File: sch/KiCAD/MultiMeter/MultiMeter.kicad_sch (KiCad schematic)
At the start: 28 parts, among them J1 Conn_01x02_Male, J2 Conn_01x02_Male, J3 Conn_01x03_Male, J4 Conn_01x03_Male, J5 Conn_01x02_Female, J6 Conn_01x15, J7 Conn_01x15, J8 Conn_01x08_Female, Q1 2SC1815, Q2 2SC1815

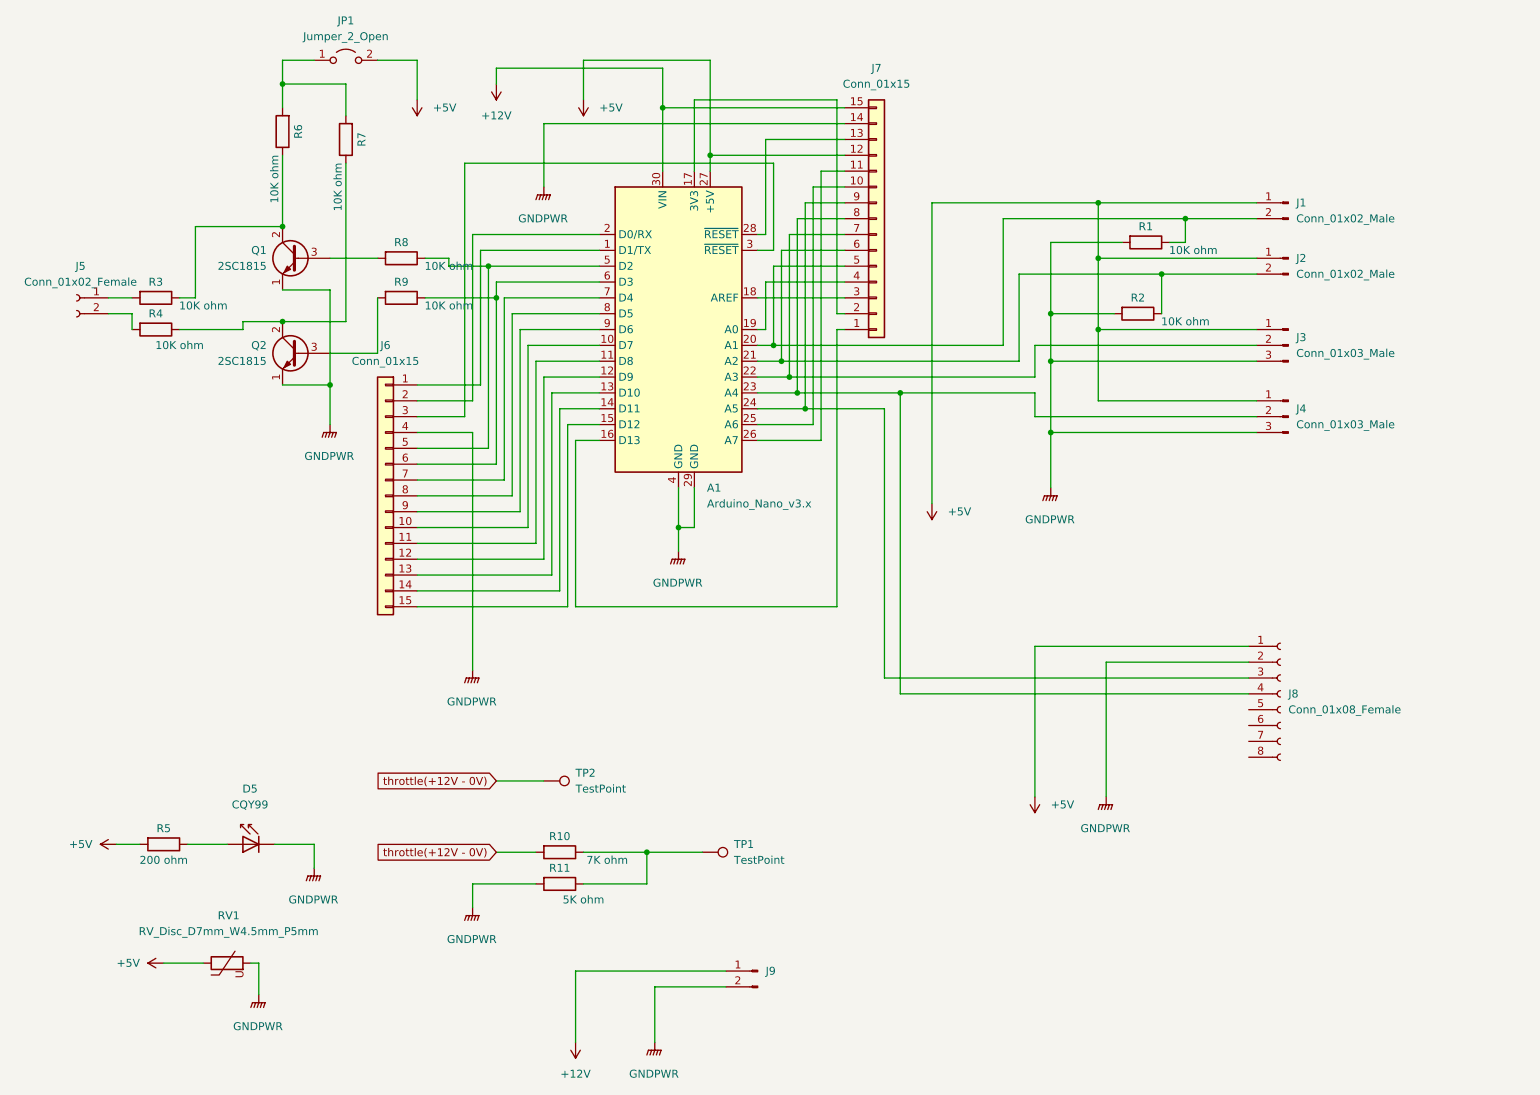
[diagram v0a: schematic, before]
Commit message: 回路図修正
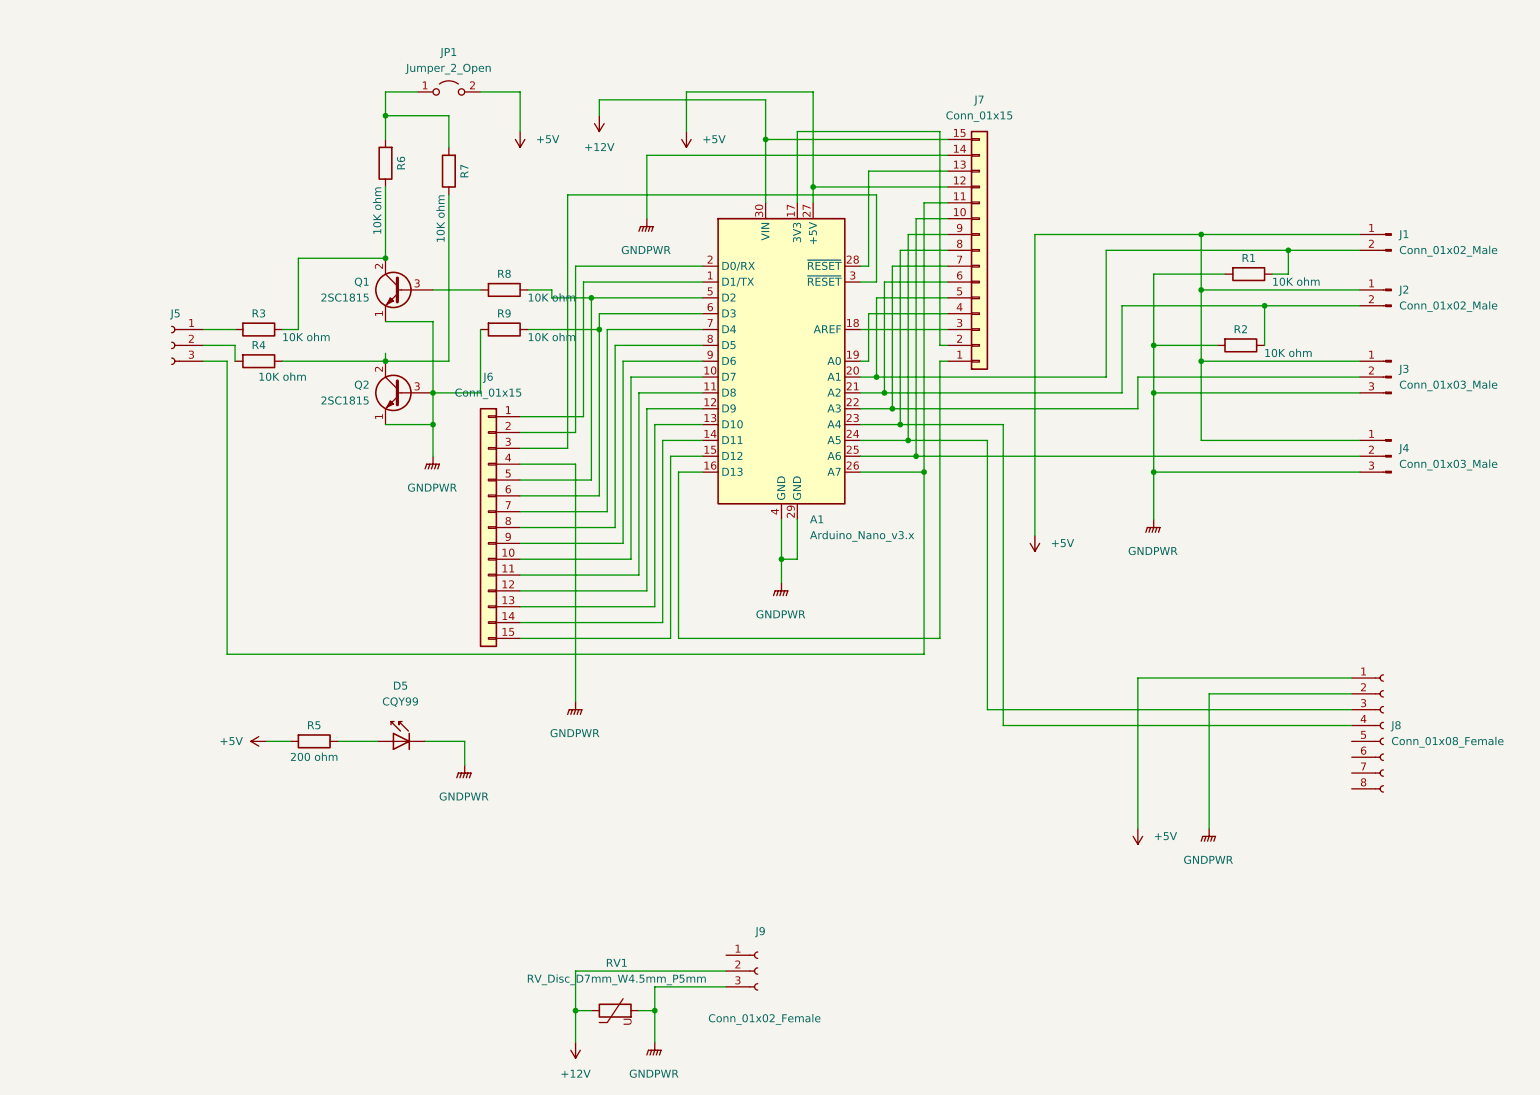
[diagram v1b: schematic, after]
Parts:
- removed R10: 7K ohm, Resistor_THT:R_Axial_DIN0204_L3.6mm_D1.6mm_P7.62mm_Horizontal, symbol Device:R
- removed R11: 5K ohm, Resistor_THT:R_Axial_DIN0204_L3.6mm_D1.6mm_P7.62mm_Horizontal, symbol Device:R
- removed TP1, TP2: TestPoint, MountingHole:MountingHole_2.2mm_M2_DIN965_Pad, symbol Connector:TestPoint
- J5: value Conn_01x02_Female -> (none); footprint Connector_Molex:Molex_KK-254_AE-6410-02A_1x02_P2.54mm_Vertical -> (none); symbol Connector:Conn_01x02_Female -> Connector:Conn_01x03_Female
- J9: value (none) -> Conn_01x02_Female; footprint (none) -> Connector_Molex:Molex_KK-254_AE-6410-02A_1x02_P2.54mm_Vertical; symbol Connector:Conn_01x02_Male -> Connector:Conn_01x03_Female
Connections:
- net +12V: now also J9.2 (Pin_2), RV1.1; no longer J9.1 (Pin_1)
- net +5V: no longer RV1.1
- net GNDPWR: now also J9.3 (Pin_3), Q2.3 (B), R9.2; no longer J9.2 (Pin_2)
- net at A1.23 (A4), J7.8 (Pin_8), J8.4 (Pin_4): no longer J4.2 (Pin_2)
- net at A1.25 (A6), J7.10 (Pin_10): now also J4.2 (Pin_2)
- net at A1.26 (A7), J7.11 (Pin_11): now also J5.3 (Pin_3)
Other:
- moved on the sheet: A1, D5, J1, J2, J3, J4, J6, J7, J8, JP1, Q1, Q2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
